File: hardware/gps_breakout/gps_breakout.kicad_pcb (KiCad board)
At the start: 2 copper layers, 33 parts, among them CON1 USB-MICRO-B, P1 CONN_01X06, P2 CONN_02X07, P3 CONN_01X03, P4 CONN_01X03, P5 CONN_01X03, U1 MCP1700, U2 CY7C65213, U3 M10478-A3

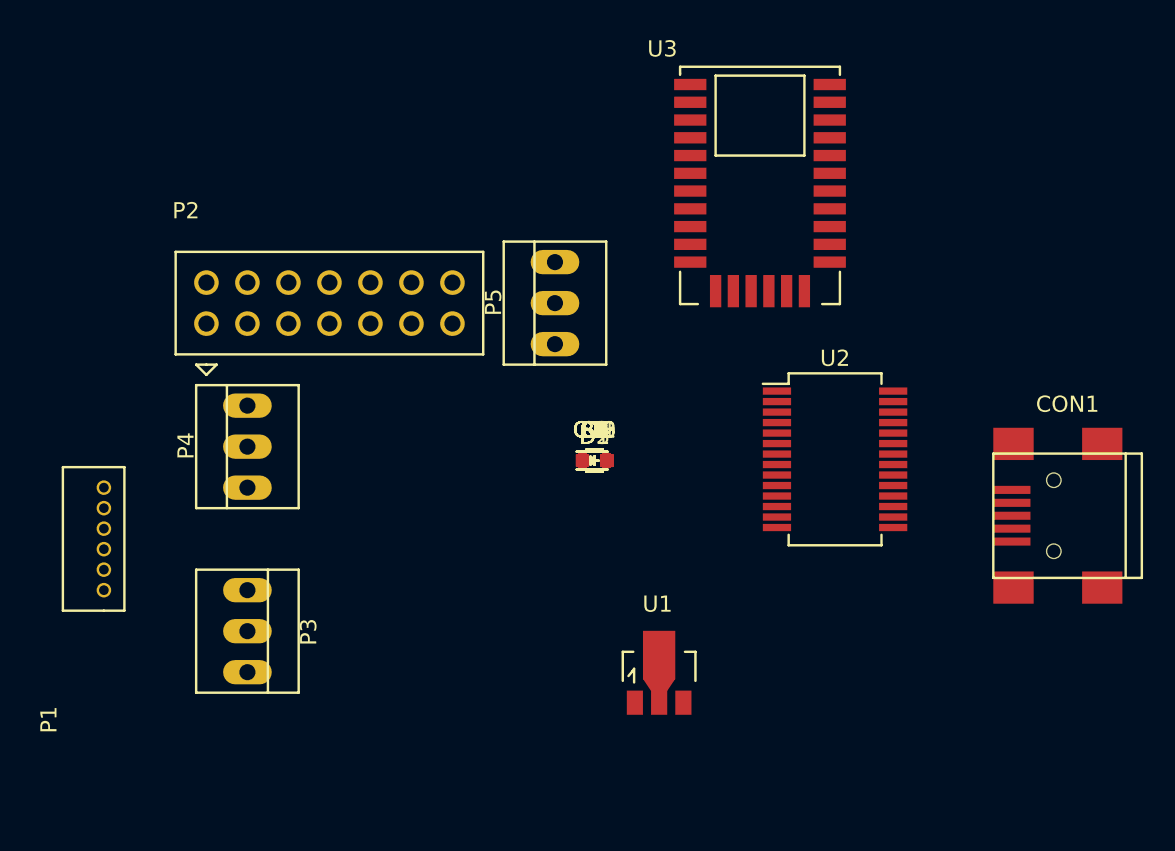
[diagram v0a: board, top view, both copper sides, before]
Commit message: finished layout of gps board
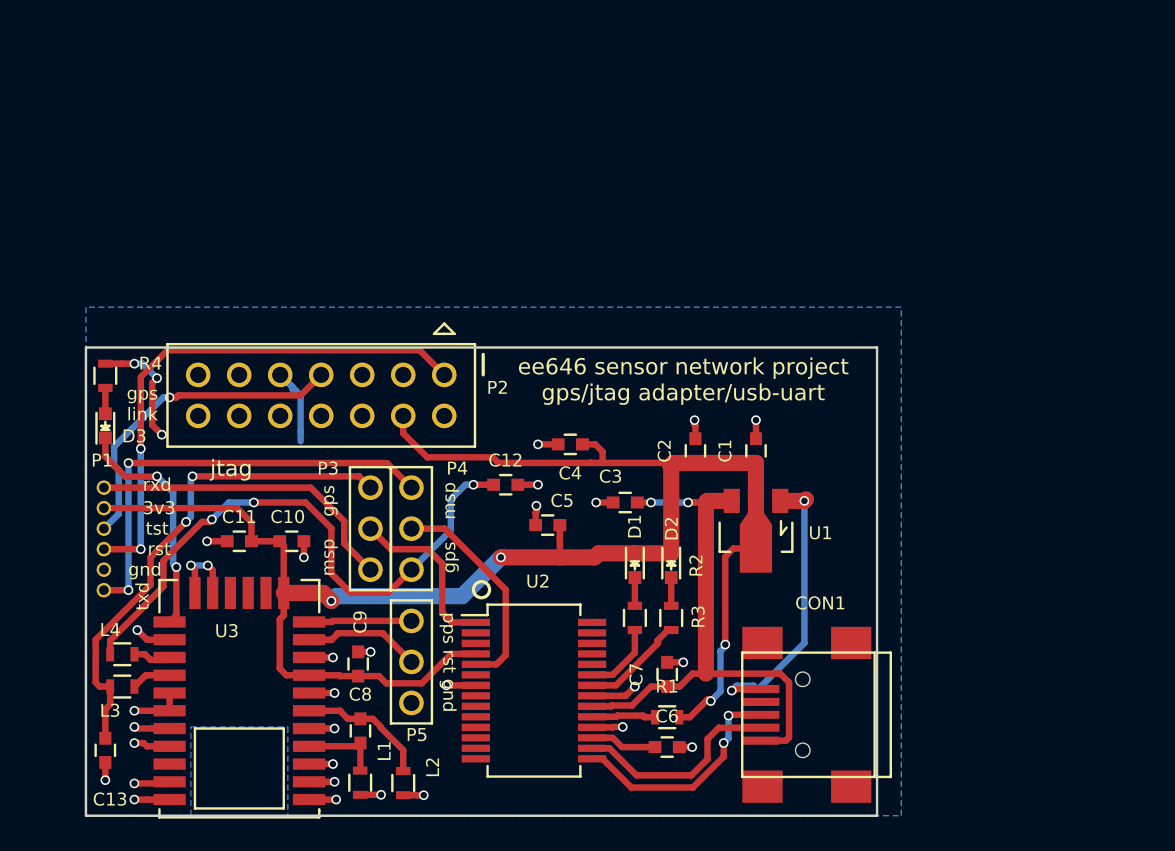
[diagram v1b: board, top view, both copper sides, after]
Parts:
- C5: value 100nF -> 1000nF
- P1: moved to B.Cu
- P3, P4, P5: footprint Connect:PINHEAD1-3 -> sensornode:JMP_HDR
- moved U3 39.2 mm to (126.5, 115.0), turned to 180 degrees
- moved C13 35.2 mm to (118.2, 123.0), turned to 270 degrees
- moved L3 32.4 mm to (119.2, 119.0), turned to 180 degrees
- moved L4 31.6 mm to (119.2, 117.0), turned to 180 degrees
- moved R4 30.8 mm to (118.2, 99.8), turned to 90 degrees
- moved D3 30.4 mm to (118.2, 102.9), turned to 90 degrees
- moved L1 24.7 mm to (134.0, 125.0), turned to 90 degrees
- moved P5 23.9 mm to (137.2, 117.5)
- moved U2 23.5 mm to (144.8, 119.2)
- moved L2 23.2 mm to (136.7, 125.0), turned to 90 degrees
- moved C11 22.6 mm to (126.5, 110.0), turned to 180 degrees
- moved C8 22.2 mm to (134.0, 121.8), turned to 90 degrees
- moved CON1 19.8 mm to (162.2, 120.8)
- moved C10 19.4 mm to (129.8, 110.0)
- moved C9 19.3 mm to (133.9, 117.6), turned to 90 degrees
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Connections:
- P2 pad 1: /RST -> /MSP_RST
- P2 pad 7: /TCK -> /MSP_TST
- U3 pad 10: Net-(P5-Pad3) -> Net-(P5-Pad2)
- U3 pad 11: Net-(P5-Pad2) -> Net-(P5-Pad3)
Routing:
- net +3V3: track 0.00 -> 113.3 mm, vias 0 -> 4
- net GND: track 0.00 -> 82.8 mm, vias 0 -> 36
- net /GPS_TXD: track 0.00 -> 37.0 mm, vias 0 -> 3
- net +5V: track 0.00 -> 35.4 mm, vias 0 -> 2
- net /MSP_RST: track 0.00 -> 33.1 mm, vias 0 -> 2
- net /GPS_RXD: track 0.00 -> 30.9 mm, vias 0 -> 2
- net /MSP_TXD: track 0.00 -> 27.6 mm, vias 0 -> 2
- net /MSP_TST: track 0.00 -> 20.3 mm, vias 0 -> 1
- net /MSP_RXD: track 0.00 -> 19.4 mm
- net Net-(D3-Pad1): track 0.00 -> 14.6 mm, vias 0 -> 2
- net Net-(CON1-Pad3): track 0.00 -> 14.4 mm, vias 0 -> 2
- net /CY_RXD: track 0.00 -> 13.5 mm
- net Net-(CON1-Pad2): track 0.00 -> 13.1 mm
- net /CY_TXD: track 0.00 -> 10.7 mm
- net Net-(C8-Pad2): track 0.00 -> 8.18 mm
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- added copper zone on B.Cu, net GND
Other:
- board outline added: 49 x 29 mm
- board text added: "3v3"
- board text added: "ee646 sensor network project gps/jtag adapter/usb-uart"
- board text added: "gnd"
- board text added: "gps"
- board text added: "gps link"
- board text added: "jtag"
- board text added: "msp"
- board text added: "pps rst gnd"
- board text added: "rst"
- board text added: "rxd"
- board text added: "tst"
- board text added: "txd"
